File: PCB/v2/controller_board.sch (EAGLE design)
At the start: 30 parts, among them M1 B4B-PH-K-S(LF)(SN), M2 B4B-PH-K-S(LF)(SN), M3 B4B-PH-K-S(LF)(SN), M4 B4B-PH-K-S(LF)(SN)

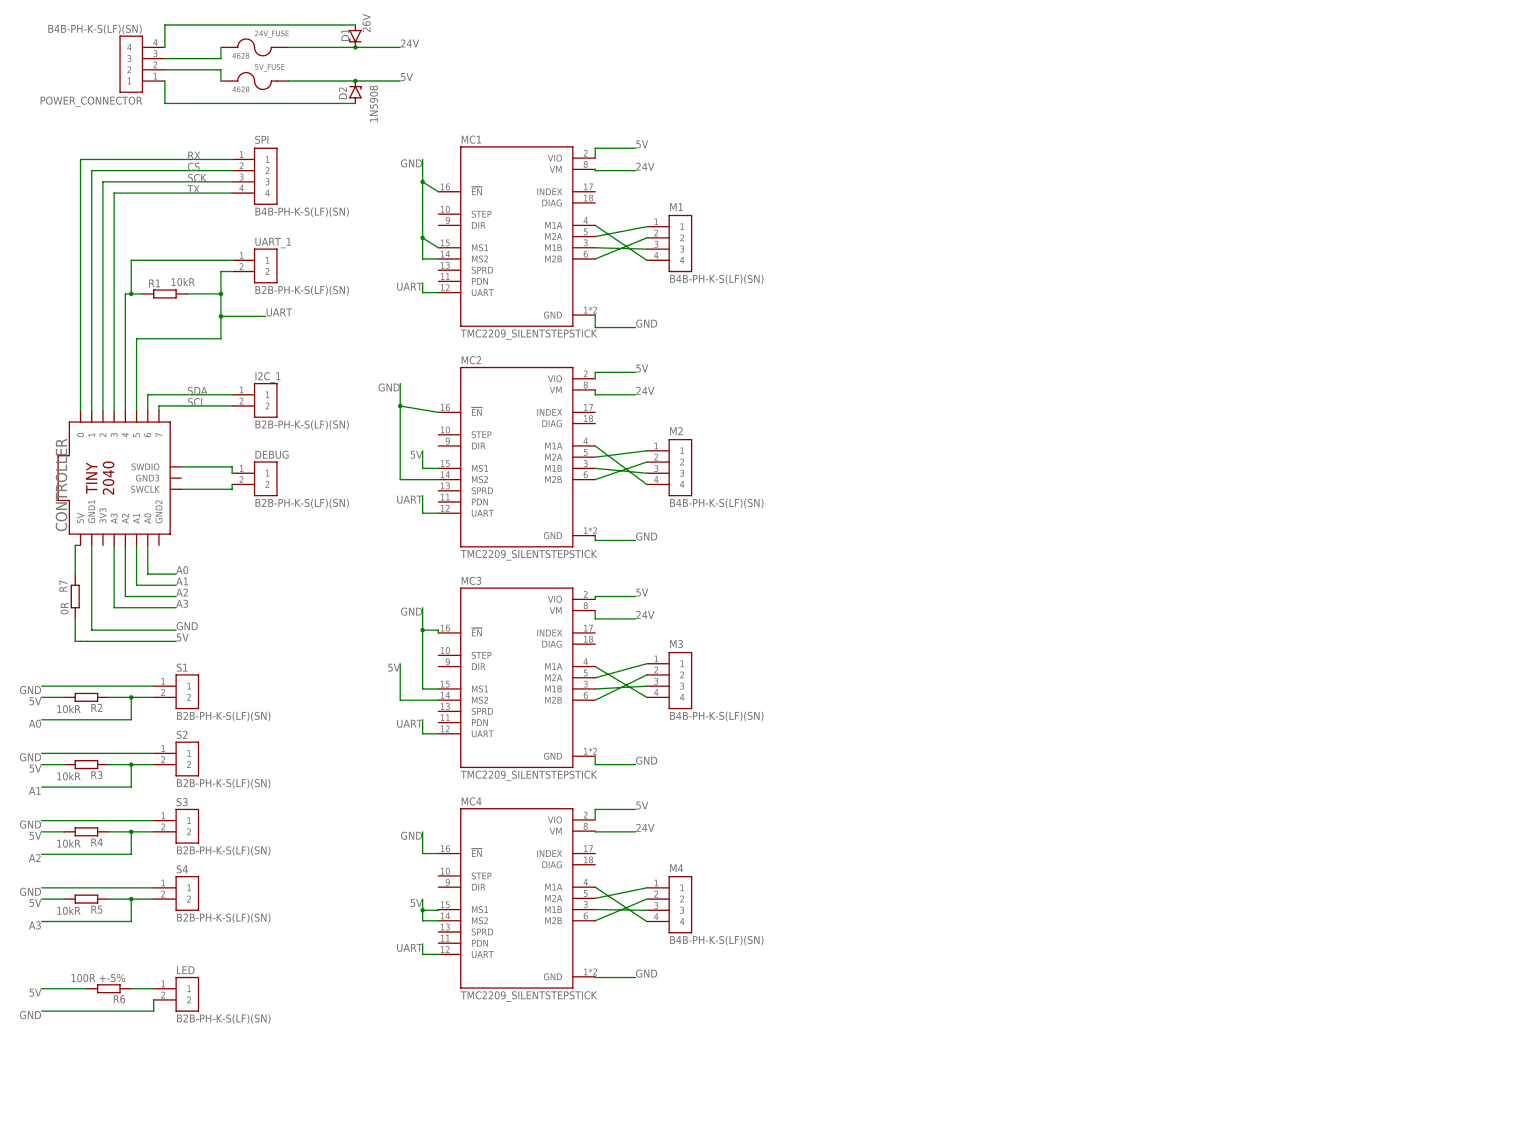
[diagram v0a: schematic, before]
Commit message: chore(pcb): improve schematics
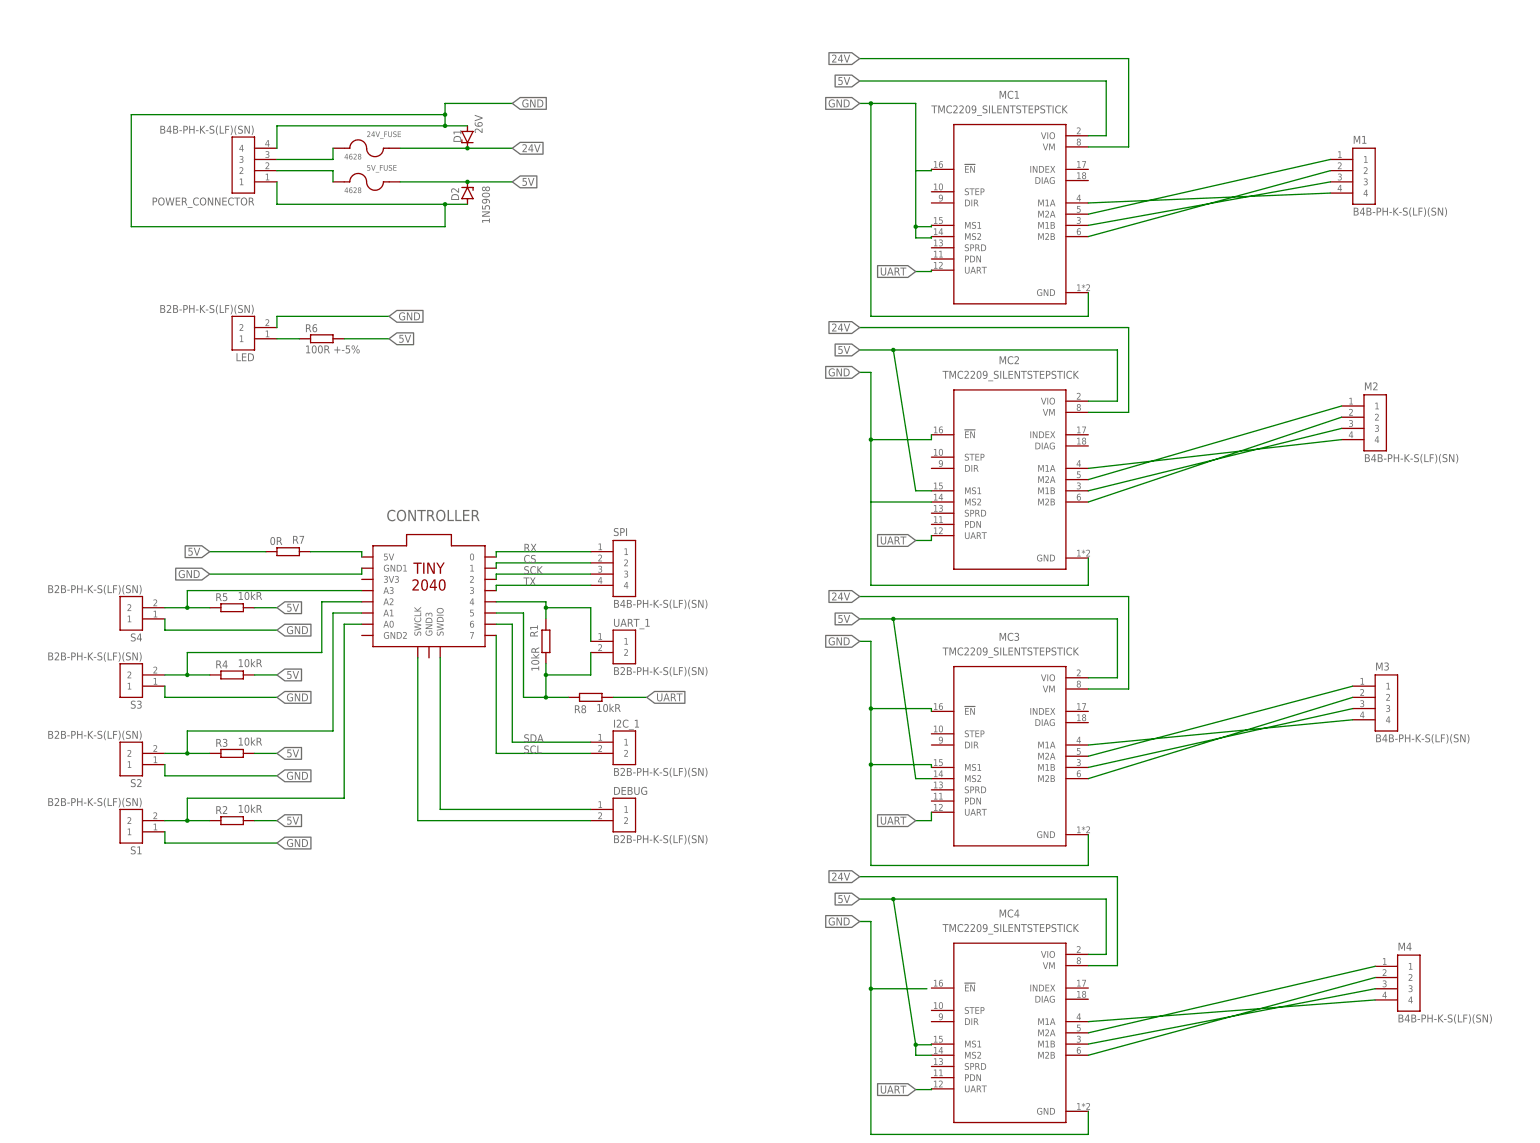
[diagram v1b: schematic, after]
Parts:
- added R8: 10kR, rcl:R-EU_R0805
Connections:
- net A3 renamed N$24
- removed net N$24 (its old number): D2.A, POWER_CONNECTOR.1
- removed net N$26: D1.A, POWER_CONNECTOR.4
- new net N$22: CONTROLLER.5, R1.2, R8.1, UART_1.2
- net GND: now also D1.A, D2.A, POWER_CONNECTOR.1, POWER_CONNECTOR.4; no longer MC4.!EN
- net UART: now also R8.2; no longer CONTROLLER.5, R1.2, UART_1.2
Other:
- moved on the sheet: 24V_FUSE, 5V_FUSE, CONTROLLER, D1, D2, DEBUG, I2C_1, LED, M1, M2, M3, M4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
